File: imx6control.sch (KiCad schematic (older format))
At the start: 11 parts

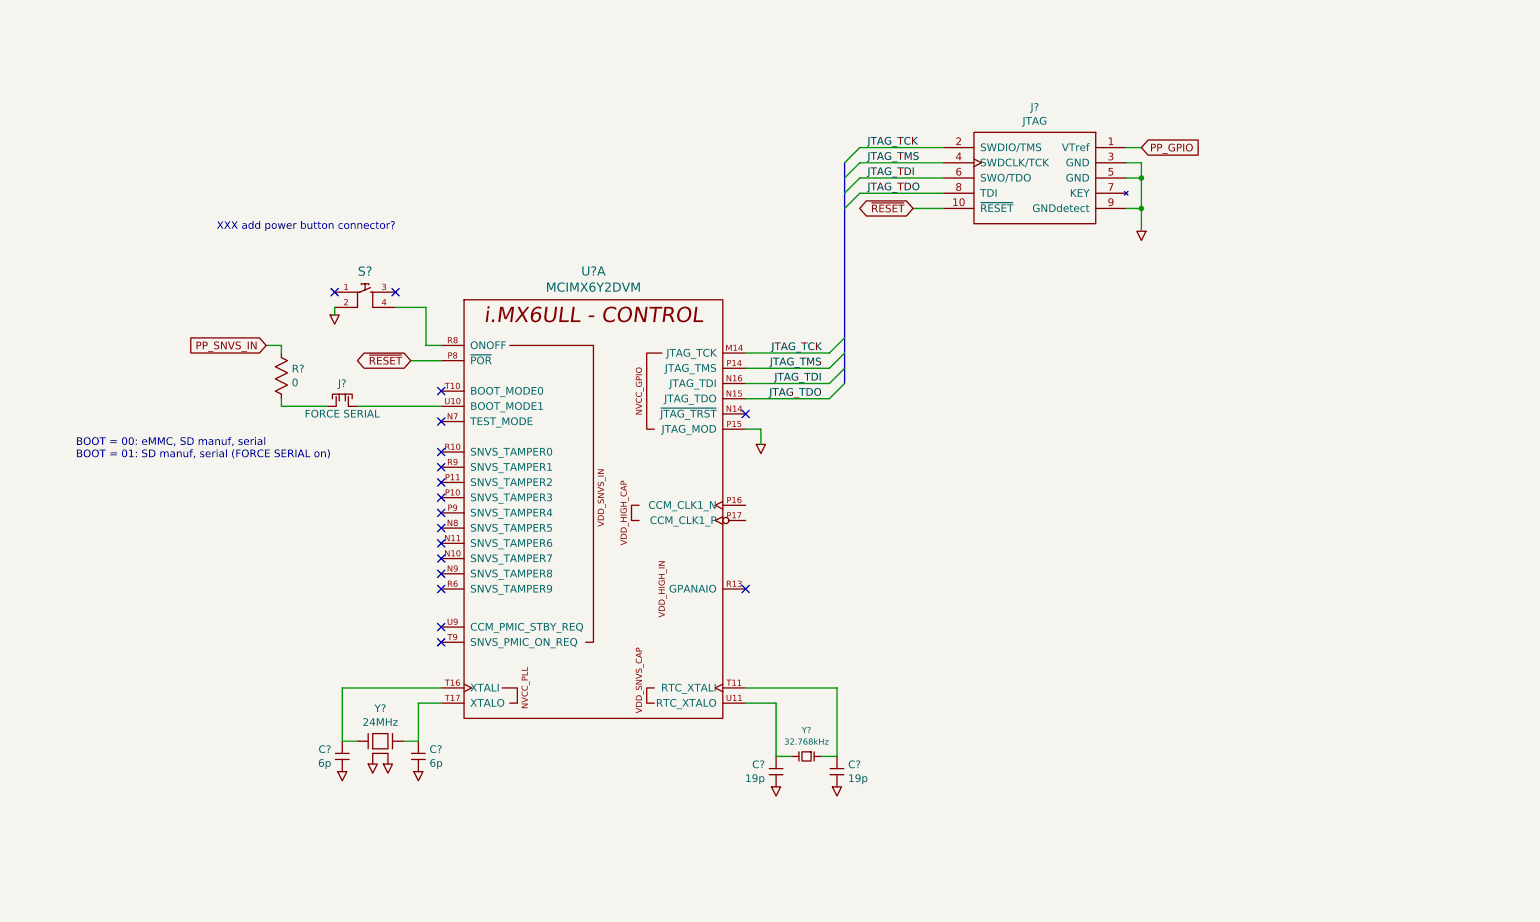
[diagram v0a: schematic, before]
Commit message: start some usb
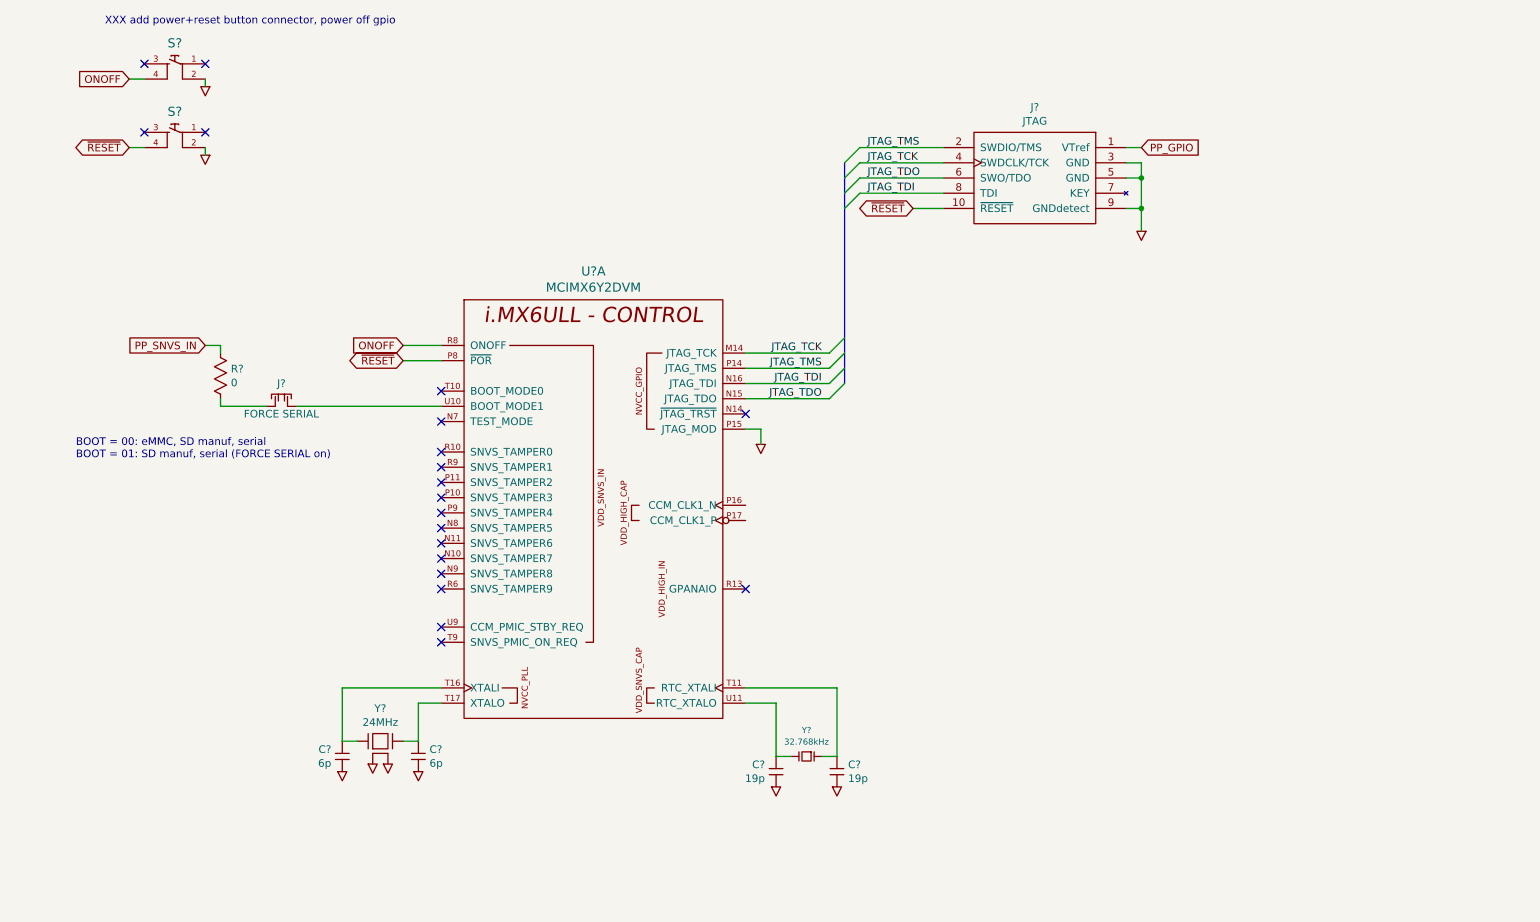
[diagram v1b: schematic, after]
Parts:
- added S?: TACTILE-4, symbol TACTILE-4
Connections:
- net COM: now also S?.2
- net JTAG_TCK: now also J?.4 (SWDCLK/TCK); no longer J?.2 (SWDIO/TMS)
- net JTAG_TDI: now also J?.8 (TDI); no longer J?.6 (SWO/TDO)
- net JTAG_TDO: now also J?.6 (SWO/TDO); no longer J?.8 (TDI)
- net JTAG_TMS: now also J?.2 (SWDIO/TMS); no longer J?.4 (SWDCLK/TCK)
- net ~RESET: now also S?.4
- net ONOFF: now reaches S?.4, U?.R8 (ONOFF)
- no-connect marks 18 -> 20
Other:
- note added: "XXX add power+reset button connector, power off gpio"
- note removed: "XXX add power button connector?"
- moved on the sheet: J?, R?, S?
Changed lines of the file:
@@
 NoConn ~ 3450 4500
 NoConn ~ 3450 4600
-Text GLabel 3250 3100 0    50   BiDi ~ 0
+Text GLabel 3200 3100 0    50   BiDi ~ 0
 ~RESET
 Wire Wire Line
-	3250 3100 3450 3100
+	3200 3100 3450 3100
 $Comp
 L JUMPER J?
 U 1 1 5A100758
-P 2800 3400
-F 0 "J?" H 2800 3550 50  0000 C CNN
-F 1 "FORCE SERIAL" H 2800 3350 50  0000 C CNN
-F 2 "" H 3100 3150 60  0000 C CNN
-F 3 "" H 3100 3150 60  0000 C CNN
-	1    2800 3400
+P 2400 3400
+F 0 "J?" H 2400 3550 50  0000 C CNN
+F 1 "FORCE SERIAL" H 2400 3350 50  0000 C CNN
+F 2 "" H 2700 3150 60  0000 C CNN
+F 3 "" H 2700 3150 60  0000 C CNN
+	1    2400 3400
 	1    0    0    -1
 $EndComp
@@
 L R R?
 U 1 1 5A100D40
-P 2400 3050
-F 0 "R?" H 2468 2946 50  0000 L CNN
-F 1 "0" H 2468 2855 50  0000 L CNN
-F 2 "" H 2535 2890 60  0000 C CNN
-F 3 "" H 2535 2890 60  0000 C CNN
-	1    2400 3050
+P 2000 3050
+F 0 "R?" H 2068 2946 50  0000 L CNN
+F 1 "0" H 2068 2855 50  0000 L CNN
+F 2 "" H 2135 2890 60  0000 C CNN
+F 3 "" H 2135 2890 60  0000 C CNN
+	1    2000 3050
 	1    0    0    -1
 $EndComp
 Wire Wire Line
-	2400 3400 2700 3400
-Text GLabel 2300 3000 0    50   Input ~ 0
+	2000 3400 2300 3400
+Text GLabel 1900 3000 0    50   Input ~ 0
 PP_SNVS_IN
 Wire Wire Line
-	2300 3000 2400 3000
-Wire Wire Line
-	2400 3000 2400 3050
-Wire Wire Line
-	2400 3350 2400 3400
-Wire Wire Line
-	2900 3400 3450 3400
+	1900 3000 2000 3000
+Wire Wire Line
+	2000 3000 2000 3050
+Wire Wire Line
+	2000 3350 2000 3400
+Wire Wire Line
+	2500 3400 3450 3400
 NoConn ~ 3450 3300
 Text Notes 1050 3750 0    50   ~ 0
@@
 	8050 2100 7950 2100
 Wire Wire Line
-	8050 1800 8050 1900
-Wire Wire Line
-	8050 1900 8050 2100
-Wire Wire Line
-	8050 2100 8050 2250
+	8050 1800 8050 2250
 Wire Wire Line
 	7950 1900 8050 1900
@@
 Wire Wire Line
 	6750 2000 6200 2000
+Text Label 6250 1900 0    50   ~ 0
+JTAG_TDO
+Wire Wire Line
+	6750 1900 6200 1900
+Wire Wire Line
+	6200 1800 6750 1800
+Wire Wire Line
+	6750 1700 6200 1700
 Text Label 6250 2000 0    50   ~ 0
-JTAG_TDO
-Wire Wire Line
-	6750 1900 6200 1900
-Wire Wire Line
-	6200 1800 6750 1800
-Wire Wire Line
-	6750 1700 6200 1700
-Text Label 6250 1900 0    50   ~ 0
 JTAG_TDI
+Text Label 6250 1700 0    50   ~ 0
+JTAG_TMS
 Text Label 6250 1800 0    50   ~ 0
-JTAG_TMS
-Text Label 6250 1700 0    50   ~ 0
 JTAG_TCK
 Entry Wire Line
@@
 	6100 1800 6200 1700
 Wire Bus Line
-	6100 1800 6100 1900
-Wire Bus Line
-	6100 1900 6100 2000
-Wire Bus Line
-	6100 2000 6100 2100
-Wire Bus Line
-	6100 2100 6100 2950
-Wire Bus Line
-	6100 2950 6100 3050
-Wire Bus Line
-	6100 3050 6100 3150
-Wire Bus Line
-	6100 3150 6100 3250
+	6100 1800 6100 3250
 $Comp
 L TACTILE-4 S?
 U 1 1 5A102FCC
-P 2950 2750
-F 0 "S?" H 2950 2986 60  0000 C CNN
-F 1 "TACTILE-4" H 2950 3000 60  0001 C CNN
-F 2 "" H 2950 2750 60  0000 C CNN
-F 3 "" H 2950 2750 60  0000 C CNN
-	1    2950 2750
-	1    0    0    -1
+P 1700 1250
+F 0 "S?" H 1700 1486 60  0000 C CNN
+F 1 "TACTILE-4" H 1700 1500 60  0001 C CNN
+F 2 "" H 1700 1250 60  0000 C CNN
+F 3 "" H 1700 1250 60  0000 C CNN
+	1    1700 1250
+	-1   0    0    -1
 $EndComp
 $Comp
 L COM #PWR?
 U 1 1 5A1030B1
-P 2750 2800
-F 0 "#PWR?" V 3025 2800 60  0001 C CNN
-F 1 "COM" H 2910 2685 30  0001 C CNN
-F 2 "" H 2905 2810 60  0000 C CNN
-F 3 "" H 2905 2810 60  0000 C CNN
-	1    2750 2800
-	1    0    0    -1
-$EndComp
-Wire Wire Line
-	2750 2750 2750 2800
-Text Notes 3150 2250 2    50   ~ 0
-XXX add power button connector?
-Wire Wire Line
-	3150 2750 3350 2750
-Wire Wire Line
-	3350 3000 3450 3000
-Wire Wire Line
-	3350 2750 3350 3000
-NoConn ~ 3150 2650
-NoConn ~ 2750 2650
+P 1900 1300
+F 0 "#PWR?" V 2175 1300 60  0001 C CNN
+F 1 "COM" H 2060 1185 30  0001 C CNN
+F 2 "" H 2055 1310 60  0000 C CNN
+F 3 "" H 2055 1310 60  0000 C CNN
+	1    1900 1300
+	-1   0    0    -1
+$EndComp
+Wire Wire Line
+	1900 1250 1900 1300
+Text Notes 3150 900  2    50   ~ 0
+XXX add power+reset button connector, power off gpio
+Wire Wire Line
+	3200 3000 3450 3000
+NoConn ~ 1500 1150
+NoConn ~ 1900 1150
+$Comp
+L TACTILE-4 S?
+U 1 1 5A104A40
+P 1700 1700
+F 0 "S?" H 1700 1936 60  0000 C CNN
+F 1 "TACTILE-4" H 1700 1950 60  0001 C CNN
+F 2 "" H 1700 1700 60  0000 C CNN
+F 3 "" H 1700 1700 60  0000 C CNN
+	1    1700 1700
+	-1   0    0    -1
+$EndComp
+Text GLabel 3200 3000 0    50   Input ~ 0
+ONOFF
+Text GLabel 1400 1250 0    50   Input ~ 0
+ONOFF
+Wire Wire Line
+	1400 1250 1500 1250
+Text GLabel 1400 1700 0    50   BiDi ~ 0
+~RESET
+Wire Wire Line
+	1400 1700 1500 1700
+NoConn ~ 1500 1600
+NoConn ~ 1900 1600
+$Comp
+L COM #PWR?
+U 1 1 5A104D16
+P 1900 1750
+F 0 "#PWR?" V 2175 1750 60  0001 C CNN
+F 1 "COM" H 2060 1635 30  0001 C CNN
+F 2 "" H 2055 1760 60  0000 C CNN
+F 3 "" H 2055 1760 60  0000 C CNN
+	1    1900 1750
+	-1   0    0    -1
+$EndComp
+Wire Wire Line
+	1900 1700 1900 1750
 $EndSCHEMATC

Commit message: schematic progress
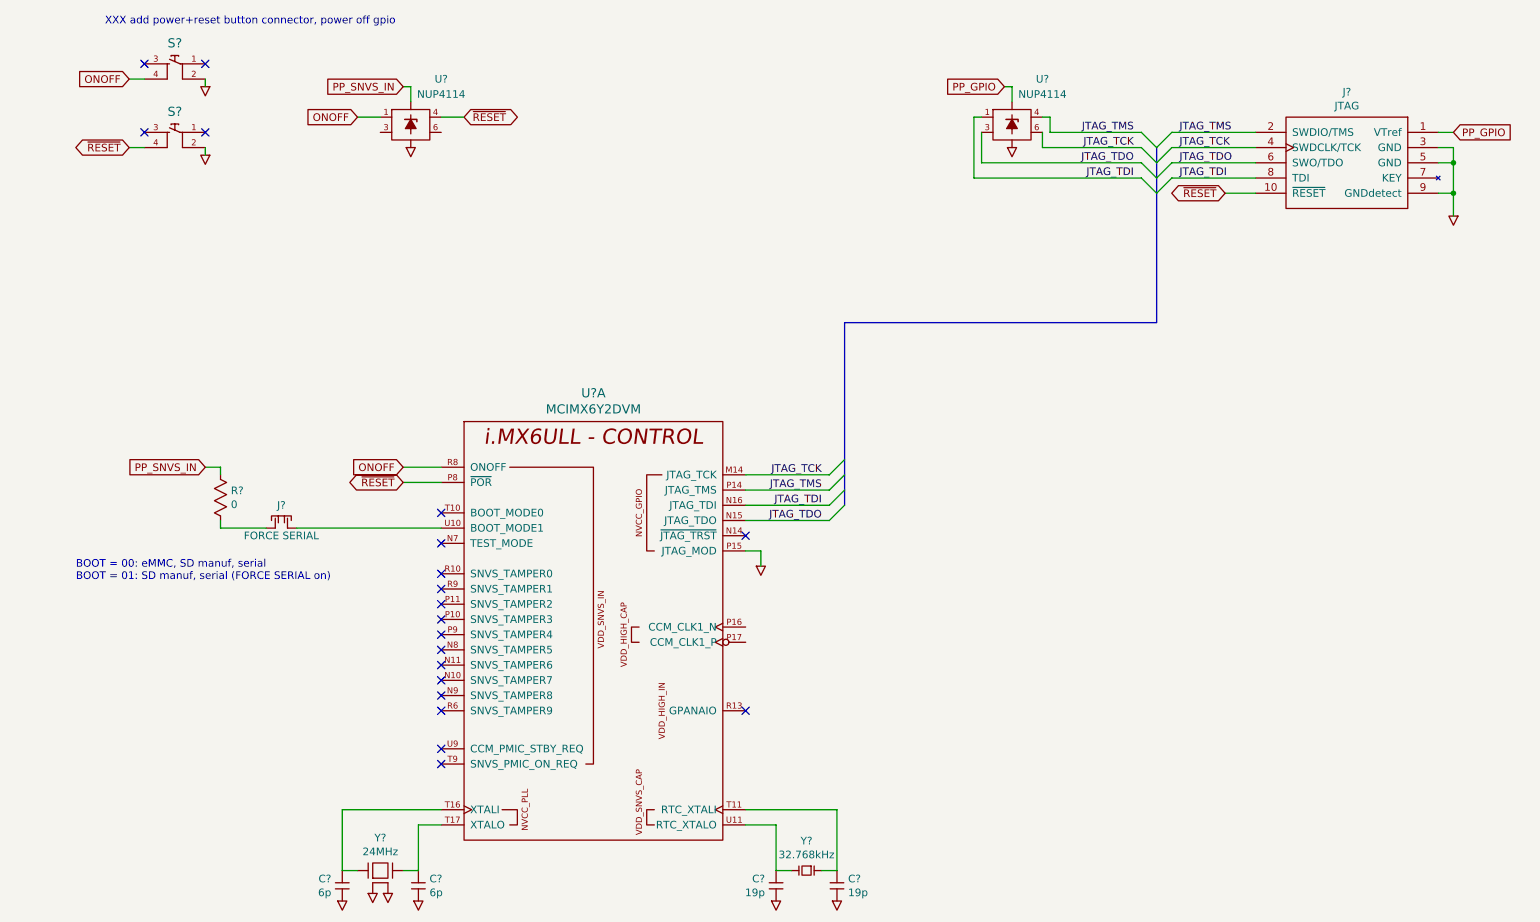
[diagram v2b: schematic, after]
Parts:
- added U? (x2): NUP4114, symbol NUP4114
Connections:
- net COM: now also U?.2, U?.2
- net JTAG_TCK: now also U?.6
- net JTAG_TDI: now also U?.1
- net JTAG_TDO: now also U?.3
- net JTAG_TMS: now also U?.4
- net ONOFF: now also U?.1
- net PP_GPIO: now also U?.5
- net PP_SNVS_IN: now also U?.5
- net ~RESET: now also U?.4
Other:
- moved on the sheet: C?, J?, R?, U?A, Y?
